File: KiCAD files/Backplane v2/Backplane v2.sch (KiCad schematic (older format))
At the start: 10 parts, among them J1 Conn_02x05_Odd_Even, J10 Conn_02x20_Odd_Even, J2 Conn_02x20_Odd_Even, J3 Conn_02x05_Odd_Even, J4 Conn_02x20_Odd_Even, J5 Conn_02x05_Odd_Even, J6 Conn_02x20_Odd_Even, J7 Conn_02x05_Odd_Even, J8 Conn_02x20_Odd_Even, J9 Conn_02x05_Odd_Even

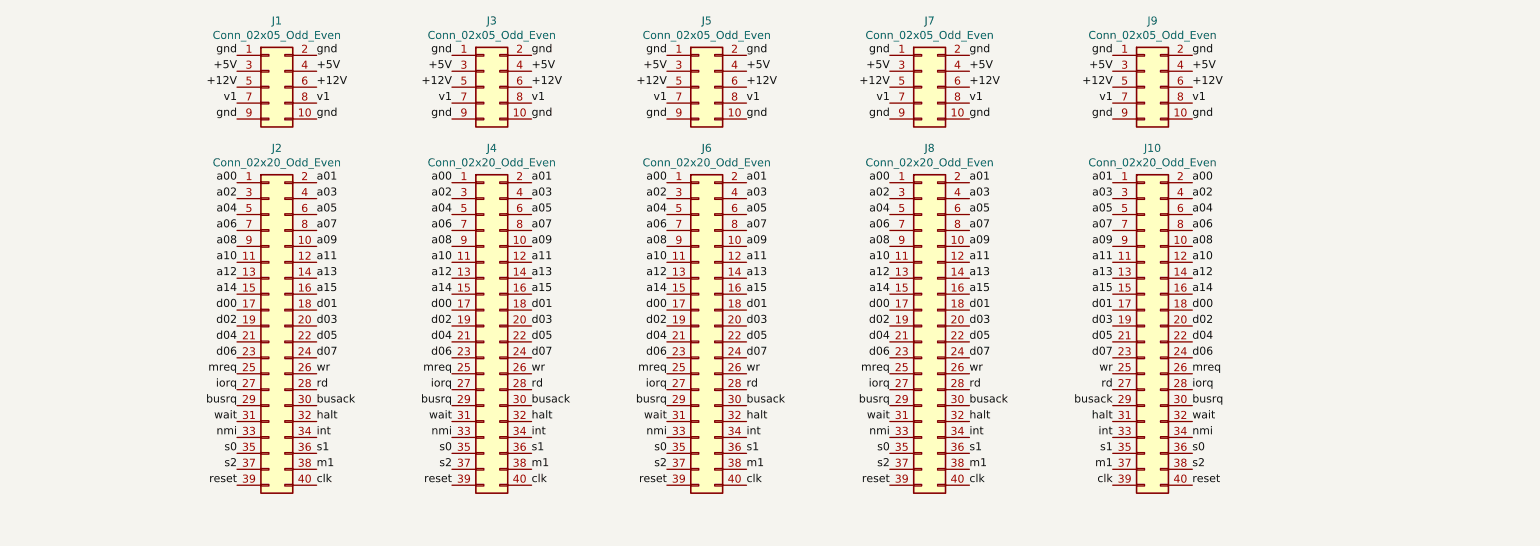
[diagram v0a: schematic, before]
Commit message: home
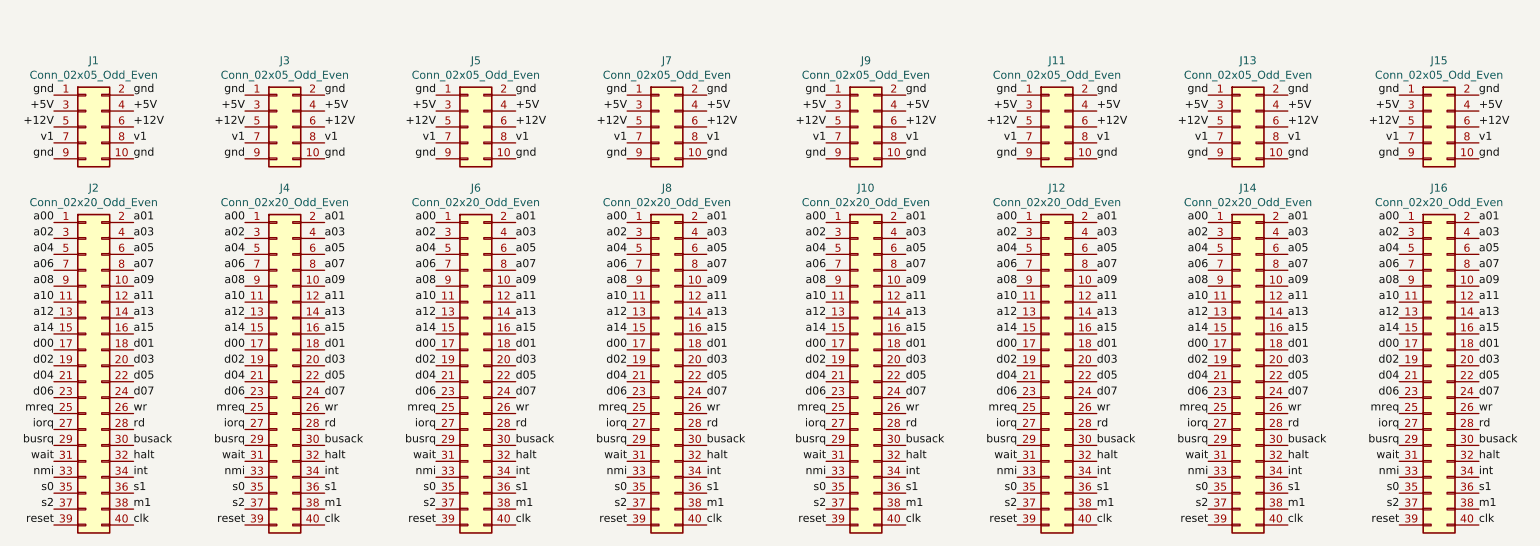
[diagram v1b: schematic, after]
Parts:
- added J11, J13, J15: Conn_02x05_Odd_Even, Connector_PinHeader_2.54mm:PinHeader_2x05_P2.54mm_Vertical, symbol Connector_Generic:Conn_02x05_Odd_Even
- added J12, J14, J16: Conn_02x20_Odd_Even, Connector_PinHeader_2.54mm:PinHeader_2x20_P2.54mm_Vertical, symbol Connector_Generic:Conn_02x20_Odd_Even
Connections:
- net +12V: now also J11.5 (Pin_5), J11.6 (Pin_6), J13.5 (Pin_5), J13.6 (Pin_6), J15.5 (Pin_5), J15.6 (Pin_6)
- net +5V: now also J11.3 (Pin_3), J11.4 (Pin_4), J13.3 (Pin_3), J13.4 (Pin_4), J15.3 (Pin_3), J15.4 (Pin_4)
- net a00: now also J10.1 (Pin_1), J12.1 (Pin_1), J14.1 (Pin_1), J16.1 (Pin_1); no longer J10.2 (Pin_2)
- net a01: now also J10.2 (Pin_2), J12.2 (Pin_2), J14.2 (Pin_2), J16.2 (Pin_2); no longer J10.1 (Pin_1)
- net a02: now also J10.3 (Pin_3), J12.3 (Pin_3), J14.3 (Pin_3), J16.3 (Pin_3); no longer J10.4 (Pin_4)
- net a03: now also J10.4 (Pin_4), J12.4 (Pin_4), J14.4 (Pin_4), J16.4 (Pin_4); no longer J10.3 (Pin_3)
- net a04: now also J10.5 (Pin_5), J12.5 (Pin_5), J14.5 (Pin_5), J16.5 (Pin_5); no longer J10.6 (Pin_6)
- net a05: now also J10.6 (Pin_6), J12.6 (Pin_6), J14.6 (Pin_6), J16.6 (Pin_6); no longer J10.5 (Pin_5)
- net a06: now also J10.7 (Pin_7), J12.7 (Pin_7), J14.7 (Pin_7), J16.7 (Pin_7); no longer J10.8 (Pin_8)
- net a07: now also J10.8 (Pin_8), J12.8 (Pin_8), J14.8 (Pin_8), J16.8 (Pin_8); no longer J10.7 (Pin_7)
- net a08: now also J10.9 (Pin_9), J12.9 (Pin_9), J14.9 (Pin_9), J16.9 (Pin_9); no longer J10.10 (Pin_10)
- net a09: now also J10.10 (Pin_10), J12.10 (Pin_10), J14.10 (Pin_10), J16.10 (Pin_10); no longer J10.9 (Pin_9)
- net a10: now also J10.11 (Pin_11), J12.11 (Pin_11), J14.11 (Pin_11), J16.11 (Pin_11); no longer J10.12 (Pin_12)
- net a11: now also J10.12 (Pin_12), J12.12 (Pin_12), J14.12 (Pin_12), J16.12 (Pin_12); no longer J10.11 (Pin_11)
- net a12: now also J10.13 (Pin_13), J12.13 (Pin_13), J14.13 (Pin_13), J16.13 (Pin_13); no longer J10.14 (Pin_14)
- net a13: now also J10.14 (Pin_14), J12.14 (Pin_14), J14.14 (Pin_14), J16.14 (Pin_14); no longer J10.13 (Pin_13)
- net a14: now also J10.15 (Pin_15), J12.15 (Pin_15), J14.15 (Pin_15), J16.15 (Pin_15); no longer J10.16 (Pin_16)
- net a15: now also J10.16 (Pin_16), J12.16 (Pin_16), J14.16 (Pin_16), J16.16 (Pin_16); no longer J10.15 (Pin_15)
- net busack: now also J10.30 (Pin_30), J12.30 (Pin_30), J14.30 (Pin_30), J16.30 (Pin_30); no longer J10.29 (Pin_29)
- net busrq: now also J10.29 (Pin_29), J12.29 (Pin_29), J14.29 (Pin_29), J16.29 (Pin_29); no longer J10.30 (Pin_30)
- net clk: now also J10.40 (Pin_40), J12.40 (Pin_40), J14.40 (Pin_40), J16.40 (Pin_40); no longer J10.39 (Pin_39)
- net d00: now also J10.17 (Pin_17), J12.17 (Pin_17), J14.17 (Pin_17), J16.17 (Pin_17); no longer J10.18 (Pin_18)
- net d01: now also J10.18 (Pin_18), J12.18 (Pin_18), J14.18 (Pin_18), J16.18 (Pin_18); no longer J10.17 (Pin_17)
- net d02: now also J10.19 (Pin_19), J12.19 (Pin_19), J14.19 (Pin_19), J16.19 (Pin_19); no longer J10.20 (Pin_20)
- net d03: now also J10.20 (Pin_20), J12.20 (Pin_20), J14.20 (Pin_20), J16.20 (Pin_20); no longer J10.19 (Pin_19)
- net d04: now also J10.21 (Pin_21), J12.21 (Pin_21), J14.21 (Pin_21), J16.21 (Pin_21); no longer J10.22 (Pin_22)
- net d05: now also J10.22 (Pin_22), J12.22 (Pin_22), J14.22 (Pin_22), J16.22 (Pin_22); no longer J10.21 (Pin_21)
- net d06: now also J10.23 (Pin_23), J12.23 (Pin_23), J14.23 (Pin_23), J16.23 (Pin_23); no longer J10.24 (Pin_24)
- net d07: now also J10.24 (Pin_24), J12.24 (Pin_24), J14.24 (Pin_24), J16.24 (Pin_24); no longer J10.23 (Pin_23)
- net gnd: now also J11.1 (Pin_1), J11.10 (Pin_10), J11.2 (Pin_2), J11.9 (Pin_9), J13.1 (Pin_1), J13.10 (Pin_10), J13.2 (Pin_2), J13.9 (Pin_9), J15.1 (Pin_1), J15.10 (Pin_10), J15.2 (Pin_2), J15.9 (Pin_9)
- net halt: now also J10.32 (Pin_32), J12.32 (Pin_32), J14.32 (Pin_32), J16.32 (Pin_32); no longer J10.31 (Pin_31)
- net int: now also J10.34 (Pin_34), J12.34 (Pin_34), J14.34 (Pin_34), J16.34 (Pin_34); no longer J10.33 (Pin_33)
- net iorq: now also J10.27 (Pin_27), J12.27 (Pin_27), J14.27 (Pin_27), J16.27 (Pin_27); no longer J10.28 (Pin_28)
- net m1: now also J10.38 (Pin_38), J12.38 (Pin_38), J14.38 (Pin_38), J16.38 (Pin_38); no longer J10.37 (Pin_37)
- net mreq: now also J10.25 (Pin_25), J12.25 (Pin_25), J14.25 (Pin_25), J16.25 (Pin_25); no longer J10.26 (Pin_26)
- net nmi: now also J10.33 (Pin_33), J12.33 (Pin_33), J14.33 (Pin_33), J16.33 (Pin_33); no longer J10.34 (Pin_34)
- net rd: now also J10.28 (Pin_28), J12.28 (Pin_28), J14.28 (Pin_28), J16.28 (Pin_28); no longer J10.27 (Pin_27)
- net reset: now also J10.39 (Pin_39), J12.39 (Pin_39), J14.39 (Pin_39), J16.39 (Pin_39); no longer J10.40 (Pin_40)
- net s0: now also J10.35 (Pin_35), J12.35 (Pin_35), J14.35 (Pin_35), J16.35 (Pin_35); no longer J10.36 (Pin_36)
- net s1: now also J10.36 (Pin_36), J12.36 (Pin_36), J14.36 (Pin_36), J16.36 (Pin_36); no longer J10.35 (Pin_35)
- net s2: now also J10.37 (Pin_37), J12.37 (Pin_37), J14.37 (Pin_37), J16.37 (Pin_37); no longer J10.38 (Pin_38)
- net v1: now also J11.7 (Pin_7), J11.8 (Pin_8), J13.7 (Pin_7), J13.8 (Pin_8), J15.7 (Pin_7), J15.8 (Pin_8)
- net wait: now also J10.31 (Pin_31), J12.31 (Pin_31), J14.31 (Pin_31), J16.31 (Pin_31); no longer J10.32 (Pin_32)
- net wr: now also J10.26 (Pin_26), J12.26 (Pin_26), J14.26 (Pin_26), J16.26 (Pin_26); no longer J10.25 (Pin_25)
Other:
- moved on the sheet: J1, J2, J3, J4, J5, J6, J7, J8
